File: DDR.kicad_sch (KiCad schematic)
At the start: 1 part

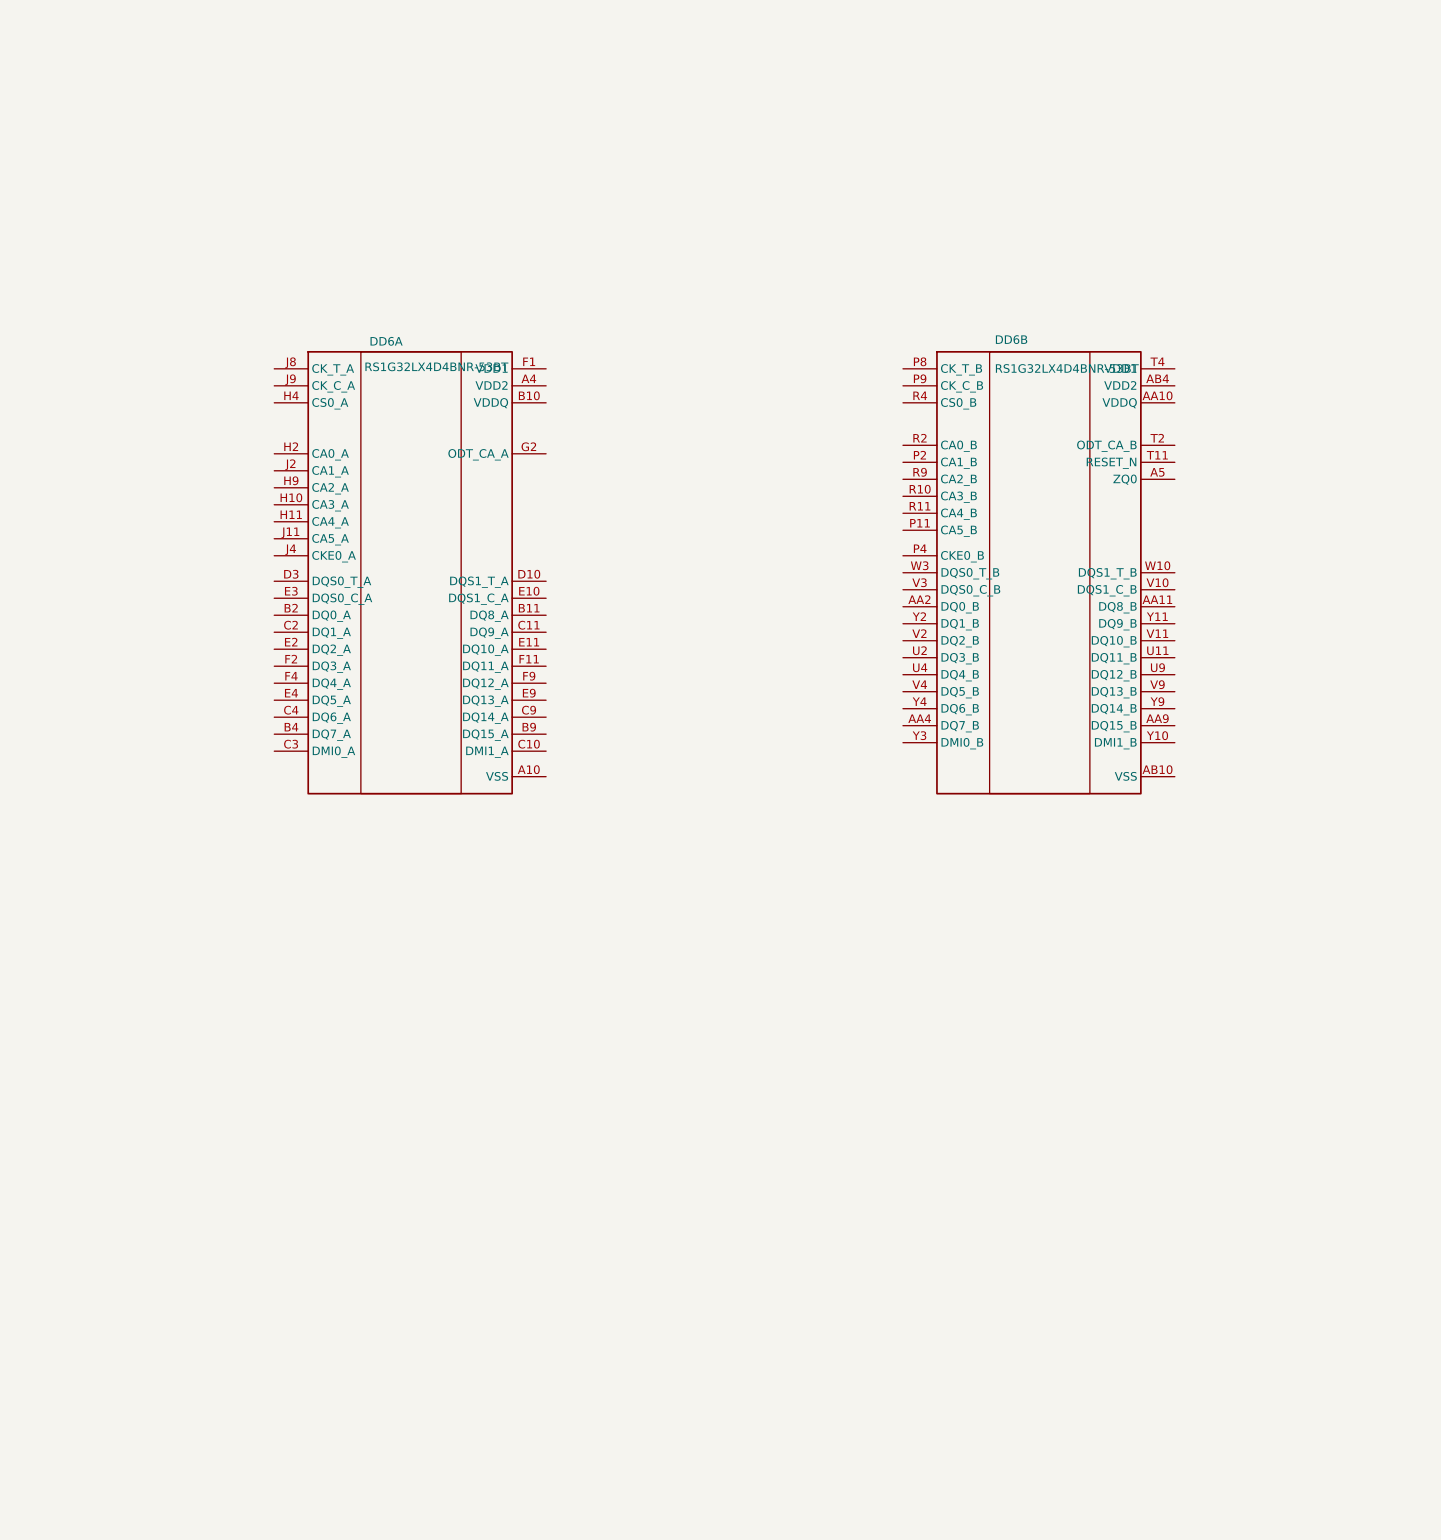
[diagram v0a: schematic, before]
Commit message: ddr
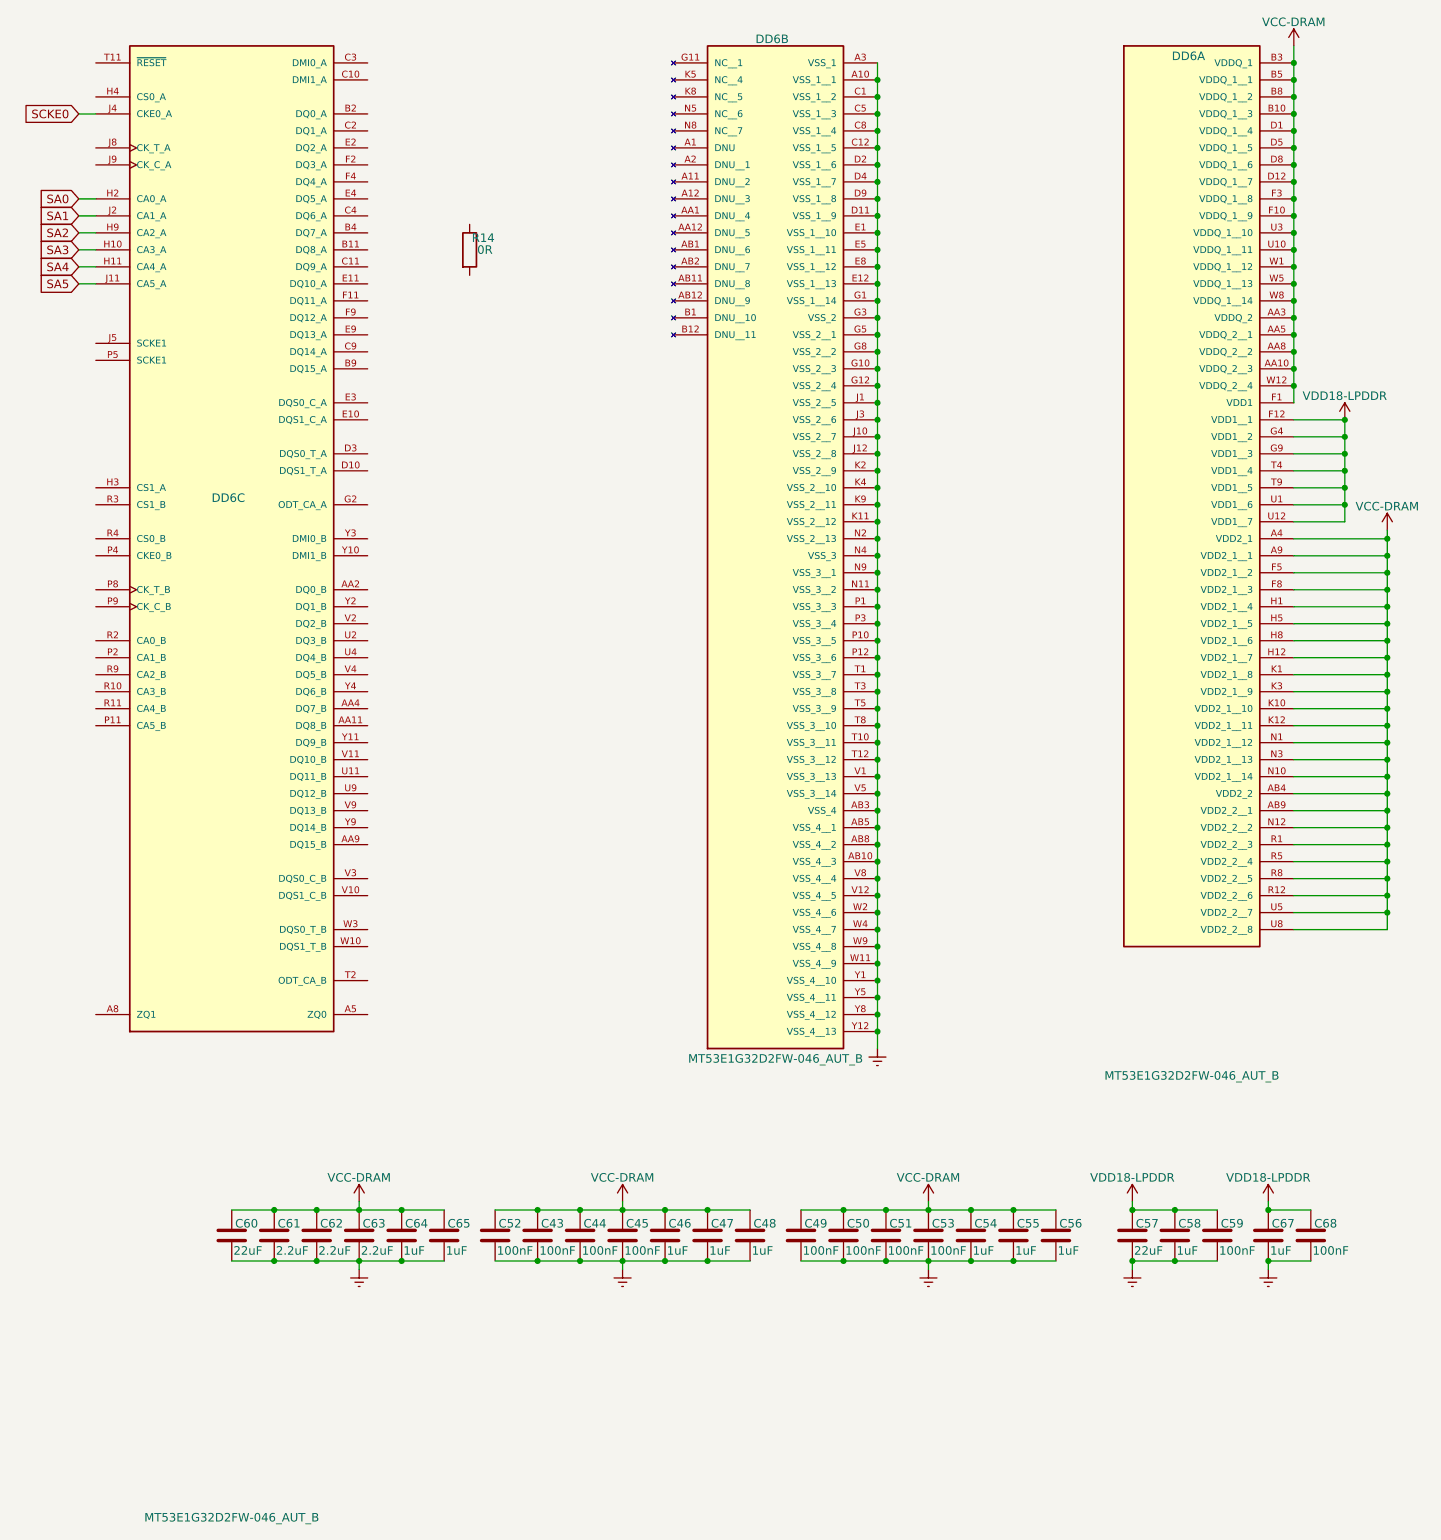
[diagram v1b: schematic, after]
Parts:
- removed DD6: RS1G32LX4D4BNR-53BT, Package_BGA:BGA-200_10.0x14.5mm_Layout12x22_P0.80x0.65mm, symbol Memory_RAM:IS43LQ32256AL-062BLI
- added C43, C44, C45, C49, C50, C51, C52, C53, C59, C68: 100nF, Capacitor_SMD:C_0402_1005Metric, symbol Device:C
- added C46, C47, C48, C54, C55, C56, C58, C64, C65, C67: 1uF, Capacitor_SMD:C_0402_1005Metric, symbol Device:C
- added C57, C60: 22uF, Capacitor_SMD:C_0402_1005Metric, symbol Device:C
- added C61, C62, C63: 2.2uF, Capacitor_SMD:C_0402_1005Metric, symbol Device:C
- added DD6: MT53E1G32D2FW-046_AUT_B, LPDDR4:BGA200C65X80P22X12_1500X1000X114N, symbol LPDDR4:MT53E1G32D2FW-046_AUT_B
- added R14: 0R, Resistor_SMD:R_0402_1005Metric, symbol Device:R
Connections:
- new net Earth: C43.2, C44.2, C45.2, C46.2, C47.2, C48.2, C49.2, C50.2, C51.2, C52.2, C53.2, C54.2, C55.2, C56.2, C57.2, C58.2, C59.2, C60.2, C61.2, C62.2, C63.2, C64.2, C65.2, C67.2, C68.2, DD6.A10 (VSS_1__1), DD6.A3 (VSS_1), DD6.AB10 (VSS_4__3), DD6.AB3 (VSS_4), DD6.AB5 (VSS_4__1), DD6.AB8 (VSS_4__2), DD6.C1 (VSS_1__2), DD6.C12 (VSS_1__5), DD6.C5 (VSS_1__3), DD6.C8 (VSS_1__4), DD6.D11 (VSS_1__9), DD6.D2 (VSS_1__6), DD6.D4 (VSS_1__7), DD6.D9 (VSS_1__8), DD6.E1 (VSS_1__10), DD6.E12 (VSS_1__13), DD6.E5 (VSS_1__11), DD6.E8 (VSS_1__12), DD6.G1 (VSS_1__14), DD6.G10 (VSS_2__3), DD6.G12 (VSS_2__4), DD6.G3 (VSS_2), DD6.G5 (VSS_2__1), DD6.G8 (VSS_2__2), DD6.J1 (VSS_2__5), DD6.J10 (VSS_2__7), DD6.J12 (VSS_2__8), DD6.J3 (VSS_2__6), DD6.K11 (VSS_2__12), DD6.K2 (VSS_2__9), DD6.K4 (VSS_2__10), DD6.K9 (VSS_2__11), DD6.N11 (VSS_3__2), DD6.N2 (VSS_2__13), DD6.N4 (VSS_3), DD6.N9 (VSS_3__1), DD6.P1 (VSS_3__3), DD6.P10 (VSS_3__5), DD6.P12 (VSS_3__6), DD6.P3 (VSS_3__4), DD6.T1 (VSS_3__7), DD6.T10 (VSS_3__11), DD6.T12 (VSS_3__12), DD6.T3 (VSS_3__8), DD6.T5 (VSS_3__9), DD6.T8 (VSS_3__10), DD6.V1 (VSS_3__13), DD6.V12 (VSS_4__5), DD6.V5 (VSS_3__14), DD6.V8 (VSS_4__4), DD6.W11 (VSS_4__9), DD6.W2 (VSS_4__6), DD6.W4 (VSS_4__7), DD6.W9 (VSS_4__8), DD6.Y1 (VSS_4__10), DD6.Y12 (VSS_4__13), DD6.Y5 (VSS_4__11), DD6.Y8 (VSS_4__12)
- new net SA0: DD6.H2 (CA0_A)
- new net SA1: DD6.J2 (CA1_A)
- new net SA2: DD6.H9 (CA2_A)
- new net SA3: DD6.H10 (CA3_A)
- new net SA4: DD6.H11 (CA4_A)
- new net SA5: DD6.J11 (CA5_A)
- new net SCKE0: DD6.J4 (CKE0_A)
- new net VCC-DRAM: C43.1, C44.1, C45.1, C46.1, C47.1, C48.1, C49.1, C50.1, C51.1, C52.1, C53.1, C54.1, C55.1, C56.1, C60.1, C61.1, C62.1, C63.1, C64.1, C65.1, DD6.A4 (VDD2_1), DD6.A9 (VDD2_1__1), DD6.AA10 (VDDQ_2__3), DD6.AA3 (VDDQ_2), DD6.AA5 (VDDQ_2__1), DD6.AA8 (VDDQ_2__2), DD6.AB4 (VDD2_2), DD6.AB9 (VDD2_2__1), DD6.B10 (VDDQ_1__3), DD6.B3 (VDDQ_1), DD6.B5 (VDDQ_1__1), DD6.B8 (VDDQ_1__2), DD6.D1 (VDDQ_1__4), DD6.D12 (VDDQ_1__7), DD6.D5 (VDDQ_1__5), DD6.D8 (VDDQ_1__6), DD6.F1 (VDD1), DD6.F10 (VDDQ_1__9), DD6.F3 (VDDQ_1__8), DD6.F5 (VDD2_1__2), DD6.F8 (VDD2_1__3), DD6.H1 (VDD2_1__4), DD6.H12 (VDD2_1__7), DD6.H5 (VDD2_1__5), DD6.H8 (VDD2_1__6), DD6.K1 (VDD2_1__8), DD6.K10 (VDD2_1__10), DD6.K12 (VDD2_1__11), DD6.K3 (VDD2_1__9), DD6.N1 (VDD2_1__12), DD6.N10 (VDD2_1__14), DD6.N12 (VDD2_2__2), DD6.N3 (VDD2_1__13), DD6.R1 (VDD2_2__3), DD6.R12 (VDD2_2__6), DD6.R5 (VDD2_2__4), DD6.R8 (VDD2_2__5), DD6.U10 (VDDQ_1__11), DD6.U3 (VDDQ_1__10), DD6.U5 (VDD2_2__7), DD6.U8 (VDD2_2__8), DD6.W1 (VDDQ_1__12), DD6.W12 (VDDQ_2__4), DD6.W5 (VDDQ_1__13), DD6.W8 (VDDQ_1__14)
- new net VDD18-LPDDR: C57.1, C58.1, C59.1, C67.1, C68.1, DD6.F12 (VDD1__1), DD6.G4 (VDD1__2), DD6.G9 (VDD1__3), DD6.T4 (VDD1__4), DD6.T9 (VDD1__5), DD6.U1 (VDD1__6), DD6.U12 (VDD1__7)
